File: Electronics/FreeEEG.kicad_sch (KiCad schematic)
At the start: 4 parts, among them J1 Electrode connector, U1 ADS131M08IPBS, U10 USBLC6-2SC6, U6 USBLC6-2SC6

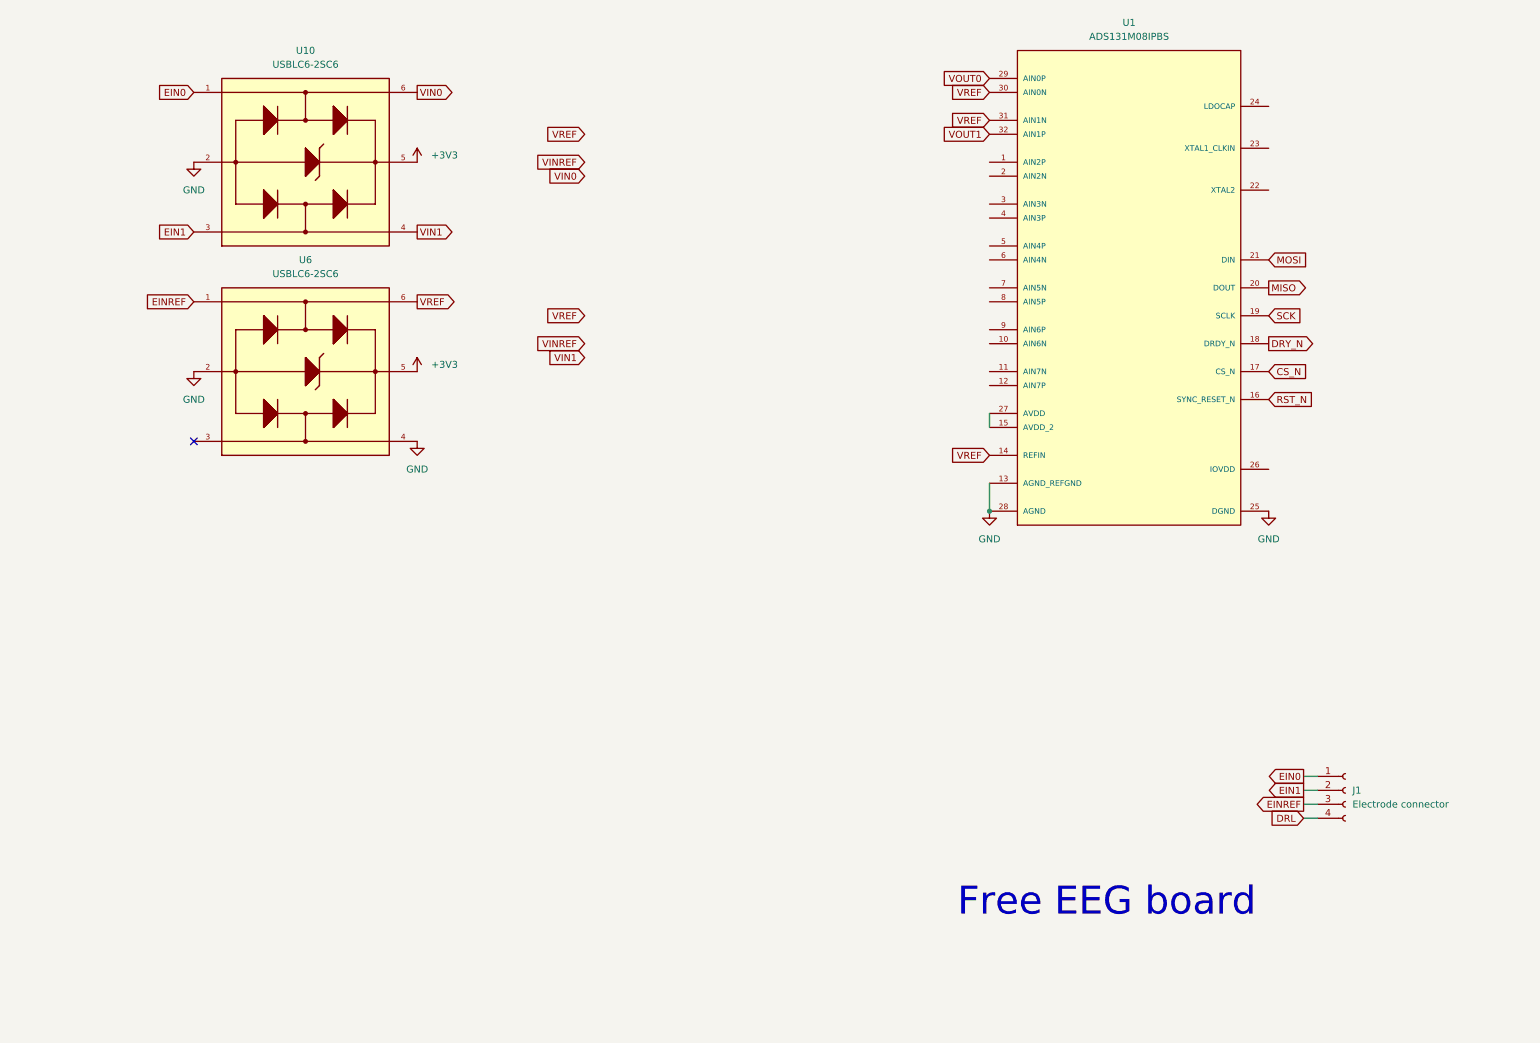
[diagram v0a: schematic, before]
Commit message: Starting final firmware development
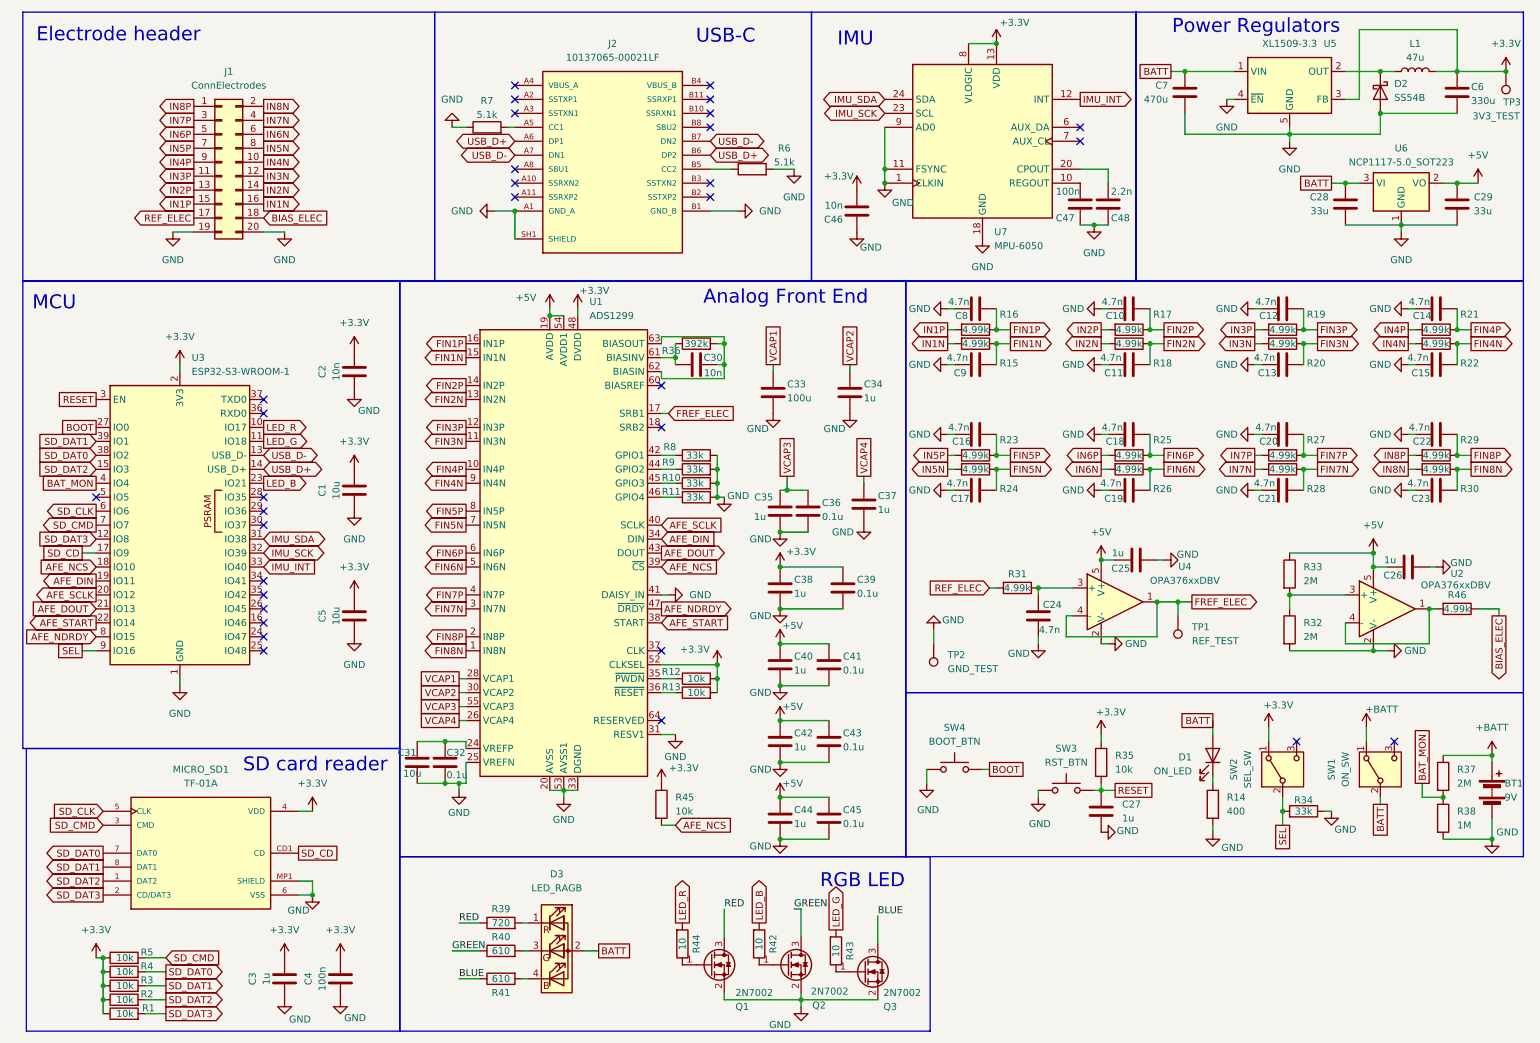
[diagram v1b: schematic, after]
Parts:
- removed J1: Electrode connector, symbol Connector:Conn_01x04_Socket
- removed U1: ADS131M08IPBS, symbol ADS131M08IPBS:ADS131M08IPBS
- removed U10, U6: USBLC6-2SC6, USBLC6-2SC6:SOT95P280X145-6N, symbol USBLC6-2SC6:USBLC6-2SC6
- added BT1: 9V, Connector_PinHeader_2.54mm:PinHeader_1x02_P2.54mm_Vertical, symbol Device:Battery
- added C1, C31, C5: 10u, Capacitor_SMD:C_0805_2012Metric, symbol Device:C
- added C10, C11, C12, C13, C14, C15, C16, C17, C18, C19, C20, C21, C22, C23, C24, C8, C9: 4.7n, Capacitor_SMD:C_0603_1608Metric, symbol Device:C
- added C2: 10n, Capacitor_SMD:C_0805_2012Metric, symbol Device:C
- added C25, C26, C27, C3: 1u, Capacitor_SMD:C_0805_2012Metric, symbol Device:C
- added C28, C29: 33u, Capacitor_SMD:C_1206_3216Metric, symbol Device:C
- added C30, C46: 10n, Capacitor_SMD:C_0603_1608Metric, symbol Device:C
- added C32, C36, C39, C41, C43, C45: 0.1u, Capacitor_SMD:C_0603_1608Metric, symbol Device:C
- added C33: 100u, Capacitor_SMD:C_Elec_6.3x7.7, symbol Device:C
- added C34, C35, C37, C38, C40, C42, C44: 1u, Capacitor_SMD:C_0603_1608Metric, symbol Device:C
- added C4: 100n, Capacitor_SMD:C_0805_2012Metric, symbol Device:C
- added C47: 100n, Capacitor_SMD:C_0603_1608Metric, symbol Device:C
- added C48: 2.2n, Capacitor_SMD:C_0603_1608Metric, symbol Device:C
- added C6: 330u, Capacitor_SMD:C_Elec_8x10.2, symbol Device:C
- added C7: 470u, Capacitor_SMD:C_Elec_8x10.2, symbol Device:C
- added D1: ON_LED, LED_SMD:LED_0805_2012Metric, symbol Device:LED
- added D2: SS54B, Diode_SMD:D_SMB, symbol Device:D_Schottky
- added D3: LED_RAGB, XL-3528RGBW-HM:XL-3528RGBW-HM, symbol Device:LED_RAGB
- added J1: ConnElectrodes, Connector_PinHeader_2.54mm:PinHeader_2x10_P2.54mm_Vertical, symbol Connector_Generic:Conn_02x10_Odd_Even
- added J2: 10137065-00021LF, 10137065-00021LF:AMPHENOL_10137065-00021LF, symbol 10137065-00021LF:10137065-00021LF
- added L1: 47u, Inductor_SMD:L_Bourns_SRP7028A_7.3x6.6mm, symbol Device:L
- added MICRO_SD1: TF-01A, TF-01A:TF-01A, symbol TF-01A:TF-01A
- added Q1, Q2, Q3: 2N7002, Package_TO_SOT_SMD:SOT-23, symbol Transistor_FET:2N7002
- added R1, R12, R13, R2, R3, R35, R4, R45, R5: 10k, Resistor_SMD:R_0603_1608Metric, symbol Device:R
- added R10, R11, R34, R8, R9: 33k, Resistor_SMD:R_0603_1608Metric, symbol Device:R
- added R14: 400, Resistor_SMD:R_0805_2012Metric, symbol Device:R
- added R15, R16, R17, R18, R19, R20, R21, R22, R23, R24, R25, R26, R27, R28, R29, R30, R31, R46: 4.99k, Resistor_SMD:R_0603_1608Metric, symbol Device:R
- added R32, R33, R37: 2M, Resistor_SMD:R_0603_1608Metric, symbol Device:R
- added R36: 392k, Resistor_SMD:R_0603_1608Metric, symbol Device:R
- added R38: 1M, Resistor_SMD:R_0603_1608Metric, symbol Device:R
- added R39: 720, Resistor_SMD:R_0805_2012Metric, symbol Device:R
- added R40, R41: 610, Resistor_SMD:R_0805_2012Metric, symbol Device:R
- added R42, R43, R44: 10, Resistor_SMD:R_0603_1608Metric, symbol Device:R
- added R6, R7: 5.1k, Resistor_SMD:R_0603_1608Metric, symbol Device:R
- added SW1: ON_SW, K3-1260D-L1:K3-1260D-L1, symbol Switch:SW_SPDT
- added SW2: SEL_SW, K3-1260D-L1:K3-1260D-L1, symbol Switch:SW_SPDT
- added SW3: RST_BTN, K2-1187SQ-A4SW-06:K2-1187SQ-A4SW-06, symbol Switch:SW_Push
- added SW4: BOOT_BTN, K2-1187SQ-A4SW-06:K2-1187SQ-A4SW-06, symbol Switch:SW_Push
- added TP1: REF_TEST, TestPoint:TestPoint_Pad_D1.5mm, symbol Connector:TestPoint
- added TP2: GND_TEST, TestPoint:TestPoint_Pad_D1.5mm, symbol Connector:TestPoint
- added TP3: 3V3_TEST, TestPoint:TestPoint_Pad_D1.5mm, symbol Connector:TestPoint
- added U1: ADS1299, Package_QFP:TQFP-64_10x10mm_P0.5mm, symbol Analog_ADC:ADS1299
- added U2, U4: OPA376xxDBV, Package_TO_SOT_SMD:SOT-23-5, symbol Amplifier_Operational:OPA376xxDBV
- added U3: ESP32-S3-WROOM-1, RF_Module:ESP32-S3-WROOM-1, symbol RF_Module:ESP32-S3-WROOM-1
- added U5: XL1509-3.3, Package_SO:SOIC-8_3.9x4.9mm_P1.27mm, symbol Regulator_Switching:XL1509-3.3
- added U6: NCP1117-5.0_SOT223, Package_TO_SOT_SMD:SOT-223-3_TabPin2, symbol Regulator_Linear:NCP1117-5.0_SOT223
- added U7: MPU-6050, Sensor_Motion:InvenSense_QFN-24_4x4mm_P0.5mm, symbol Sensor_Motion:MPU-6050
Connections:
- net GND: now also BT1.2 (-), C1.1, C10.2, C11.2, C12.2, C13.2, C14.2, C15.2, C16.2, C17.2, C18.2, C19.2, C2.2, C20.2, C21.2, C22.2, C23.2, C24.2, C25.1, C26.1, C27.2, C28.2, C29.2, C3.1, C31.2, C32.2, C33.2, C34.2, C35.2, C36.2, C37.2, C38.2, C39.2, C4.2, C40.2, C41.2, C42.2, C43.2, C44.2, C45.2, C46.1, C47.1, C48.1, C5.1, C6.2, C7.2, C8.2, C9.2, D2.2 (A), J1.19 (Pin_19), J1.20 (Pin_20), J2.A1 (GND_A), J2.A12 (GND_A), J2.B1 (GND_B), J2.B12 (GND_B), J2.SH1 (SHIELD), J2.SH2 (SHIELD), J2.SH3 (SHIELD), J2.SH4 (SHIELD), MICRO_SD1.6 (VSS), MICRO_SD1.MP1 (SHIELD), MICRO_SD1.MP2 (SHIELD), MICRO_SD1.MP3 (SHIELD), MICRO_SD1.MP4 (SHIELD), Q1.2 (S), Q2.2 (S), Q3.2 (S), R10.2, R11.2, R14.2, R32.2, R34.1, R38.2, R6.2, R7.1, R8.2, R9.2, SW3.1, SW4.1, TP2.1, U1.20 (AVSS), U1.23 (AVSS), U1.25 (VREFN), U1.31 (RESV1), U1.32 (AVSS), U1.33 (DGND), U1.41 (DAISY_IN), U1.49 (DGND), U1.51 (DGND), U1.53 (AVSS1), U1.57 (AVSS), U1.58 (AVSS), U2.2 (V-), U3.1 (GND), U3.40 (GND), U3.41 (GND), U4.2 (V-), U5.4 (~{EN}), U5.5 (GND), U5.6 (GND), U5.7 (GND), U5.8 (GND), U6.1 (GND), U7.1 (CLKIN), U7.11 (FSYNC), U7.18 (GND), U7.9 (AD0)
- new net: Q1.1 (G), R44.1
- new net: R10.1, U1.45 (GPIO3)
- new net: C30.1, R36.1, U1.61 (BIASINV)
- new net: C30.2, R36.2, U1.62 (BIASIN), U1.63 (BIASOUT)
- new net: J2.B5 (CC2), R6.1
- new net: J2.A5 (CC1), R7.2
- new net: C24.1, R31.1, U4.3 (+)
- new net: C47.2, U7.10 (REGOUT)
- new net: Q2.1 (G), R42.1
- new net: D3.1 (RK), R39.2
- new net: D3.3 (GK), R40.2
- new net: R8.1, U1.42 (GPIO1)
- new net: R32.1, R33.2, U2.3 (+)
- new net: C31.1, C32.1, U1.24 (VREFP)
- new net: C48.2, U7.20 (CPOUT)
- new net: R13.1, U1.36 (~{RESET})
- new net: R46.2, U2.1, U2.4 (-)
- new net: Q3.1 (G), R43.1
- new net: R12.1, U1.35 (~{PWDN})
- new net: R9.1, U1.44 (GPIO2)
- new net: R11.1, U1.46 (GPIO4)
- new net: D1.1 (K), R14.1
- new net: D2.1 (K), L1.1, U5.2 (OUT)
- new net: D3.4 (BK), R41.2
- new net +3.3V: C1.2, C2.1, C3.2, C38.1, C39.1, C4.1, C46.2, C5.2, C6.1, L1.2, MICRO_SD1.4 (VDD), R1.1, R12.2, R13.2, R2.1, R3.1, R35.1, R4.1, R45.1, R5.1, SW2.1 (A), TP3.1, U1.48 (DVDD), U1.50 (DVDD), U1.52 (CLKSEL), U3.2 (3V3), U5.3 (FB), U7.13 (VDD), U7.8 (VLOGIC)
- new net +5V: C25.2, C26.2, C29.1, C40.1, C41.1, C42.1, C43.1, C44.1, C45.1, R33.1, U1.19 (AVDD), U1.21 (AVDD), U1.22 (AVDD), U1.54 (AVDD1), U1.56 (AVDD), U1.59 (AVDD), U2.5 (V+), U4.5 (V+), U6.2 (VO)
- new net +BATT: BT1.1 (+), R37.1, SW1.1 (A)
- new net AFE_DIN: U1.34 (DIN), U3.19 (IO11)
- new net AFE_DOUT: U1.43 (DOUT), U3.21 (IO13)
- new net AFE_NCS: R45.2, U1.39 (~{CS}), U3.18 (IO10)
- new net AFE_NDRDY: U1.47 (~{DRDY}), U3.8 (IO15)
- new net AFE_SCLK: U1.40 (SCLK), U3.20 (IO12)
- new net AFE_START: U1.38 (START), U3.22 (IO14)
- new net BATT: C28.1, C7.1, D1.2 (A), D3.2 (A), SW1.2 (B), U5.1 (VIN), U6.3 (VI)
- new net BAT_MON: R37.2, R38.1, U3.4 (IO4)
- new net BIAS_ELEC: J1.18 (Pin_18), R46.1
- new net BLUE: Q3.3 (D), R41.1
- new net BOOT: SW4.2, U3.27 (IO0)
- new net FIN1N: C9.1, R15.1, U1.15 (IN1N)
- new net FIN1P: C8.1, R16.1, U1.16 (IN1P)
- new net FIN2N: C11.1, R18.1, U1.13 (IN2N)
- new net FIN2P: C10.1, R17.1, U1.14 (IN2P)
- new net FIN3N: C13.1, R20.1, U1.11 (IN3N)
- new net FIN3P: C12.1, R19.1, U1.12 (IN3P)
- new net FIN4N: C15.1, R22.1, U1.9 (IN4N)
- new net FIN4P: C14.1, R21.1, U1.10 (IN4P)
- new net FIN5N: C17.1, R24.1, U1.7 (IN5N)
- new net FIN5P: C16.1, R23.1, U1.8 (IN5P)
- new net FIN6N: C19.1, R26.1, U1.5 (IN6N)
- new net FIN6P: C18.1, R25.1, U1.6 (IN6P)
- new net FIN7N: C21.1, R28.1, U1.3 (IN7N)
- new net FIN7P: C20.1, R27.1, U1.4 (IN7P)
- new net FIN8N: C23.1, R30.1, U1.1 (IN8N)
- new net FIN8P: C22.1, R29.1, U1.2 (IN8P)
- new net FREF_ELEC: TP1.1, U1.17 (SRB1), U4.1, U4.4 (-)
- new net GREEN: Q2.3 (D), R40.1
- new net IMU_INT: U3.33 (IO40), U7.12 (INT)
- new net IMU_SCK: U3.32 (IO39), U7.23 (SCL)
- new net IMU_SDA: U3.31 (IO38), U7.24 (SDA)
- new net IN1N: J1.16 (Pin_16), R15.2
- new net IN1P: J1.15 (Pin_15), R16.2
- new net IN2N: J1.14 (Pin_14), R18.2
- new net IN2P: J1.13 (Pin_13), R17.2
- new net IN3N: J1.12 (Pin_12), R20.2
- new net IN3P: J1.11 (Pin_11), R19.2
- new net IN4N: J1.10 (Pin_10), R22.2
- new net IN4P: J1.9 (Pin_9), R21.2
- new net IN5N: J1.8 (Pin_8), R24.2
- new net IN5P: J1.7 (Pin_7), R23.2
- new net IN6N: J1.6 (Pin_6), R26.2
- new net IN6P: J1.5 (Pin_5), R25.2
- new net IN7N: J1.4 (Pin_4), R28.2
- new net IN7P: J1.3 (Pin_3), R27.2
- new net IN8N: J1.2 (Pin_2), R30.2
- new net IN8P: J1.1 (Pin_1), R29.2
- new net LED_B: R42.2, U3.23 (IO21)
- new net LED_G: R43.2, U3.11 (IO18)
- new net LED_R: R44.2, U3.10 (IO17)
- new net RED: Q1.3 (D), R39.1
- new net REF_ELEC: J1.17 (Pin_17), R31.2
- new net RESET: C27.1, R35.2, SW3.2, U3.3 (EN)
- new net SD_CD: MICRO_SD1.CD1 (CD), U3.17 (IO9)
- new net SD_CLK: MICRO_SD1.5 (CLK), U3.6 (IO6)
- new net SD_CMD: MICRO_SD1.3 (CMD), R5.2, U3.7 (IO7)
- new net SD_DAT0: MICRO_SD1.7 (DAT0), R4.2, U3.38 (IO2)
- new net SD_DAT1: MICRO_SD1.8 (DAT1), R3.2, U3.39 (IO1)
- new net SD_DAT2: MICRO_SD1.1 (DAT2), R2.2, U3.15 (IO3)
- new net SD_DAT3: MICRO_SD1.2 (CD/DAT3), R1.2, U3.12 (IO8)
- new net SEL: R34.2, SW2.2 (B), U3.9 (IO16)
- new net USB_D+: J2.A6 (DP1), J2.B6 (DP2), U3.14 (USB_D+)
- new net USB_D-: J2.A7 (DN1), J2.B7 (DN2), U3.13 (USB_D-)
- new net VBUS_A: J2.A4 (VBUS_A), J2.A9 (VBUS_A)
- new net VBUS_B: J2.B4 (VBUS_B), J2.B9 (VBUS_B)
- new net VCAP1: C33.1, U1.28 (VCAP1)
- new net VCAP2: C34.1, U1.30 (VCAP2)
- new net VCAP3: C35.1, C36.1, U1.55 (VCAP3)
- new net VCAP4: C37.1, U1.26 (VCAP4)
- no-connect marks 1 -> 32
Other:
- note added: "Analog Front End"
- note added: "Electrode header"
- note added: "IMU"
- note added: "MCU"
- note added: "Power Regulators"
- note added: "RGB LED"
- note added: "SD card reader"
- note added: "USB-C"
- note removed: "Free EEG board"
- title: (none) -> FreeEEG
